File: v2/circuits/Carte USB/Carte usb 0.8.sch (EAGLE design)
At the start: 15 parts, among them Q1 TIP31C, Q2 TIP31C, Q3 TIP31C, Q4 TIP30, Q5 TIP30, Q6 TIP30, X1 MKS1854-6-0-404, X2 MKS1854-6-0-404, X3 MKS1854-6-0-404

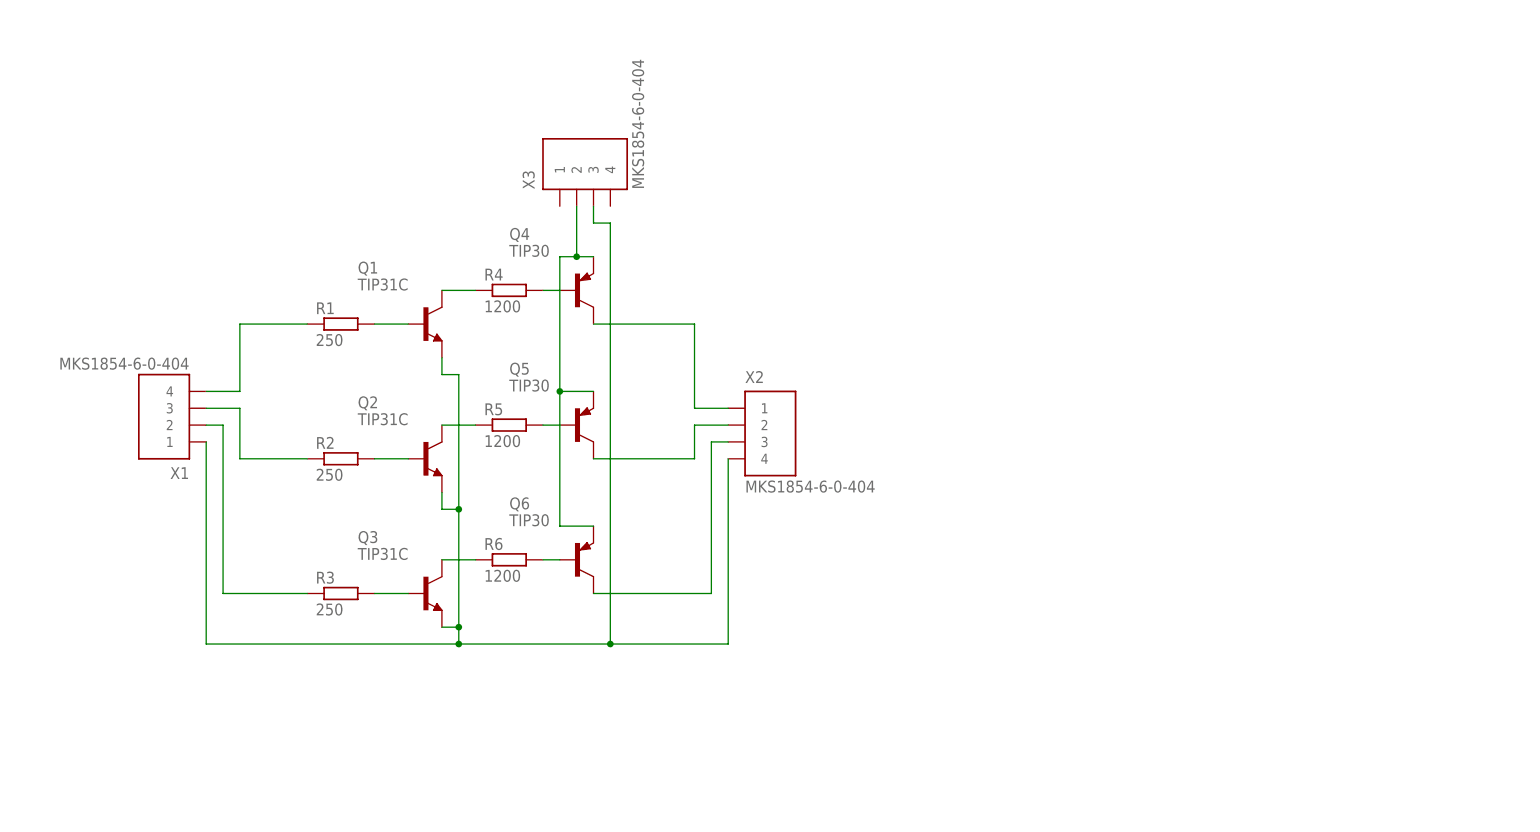
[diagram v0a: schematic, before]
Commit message: added boards
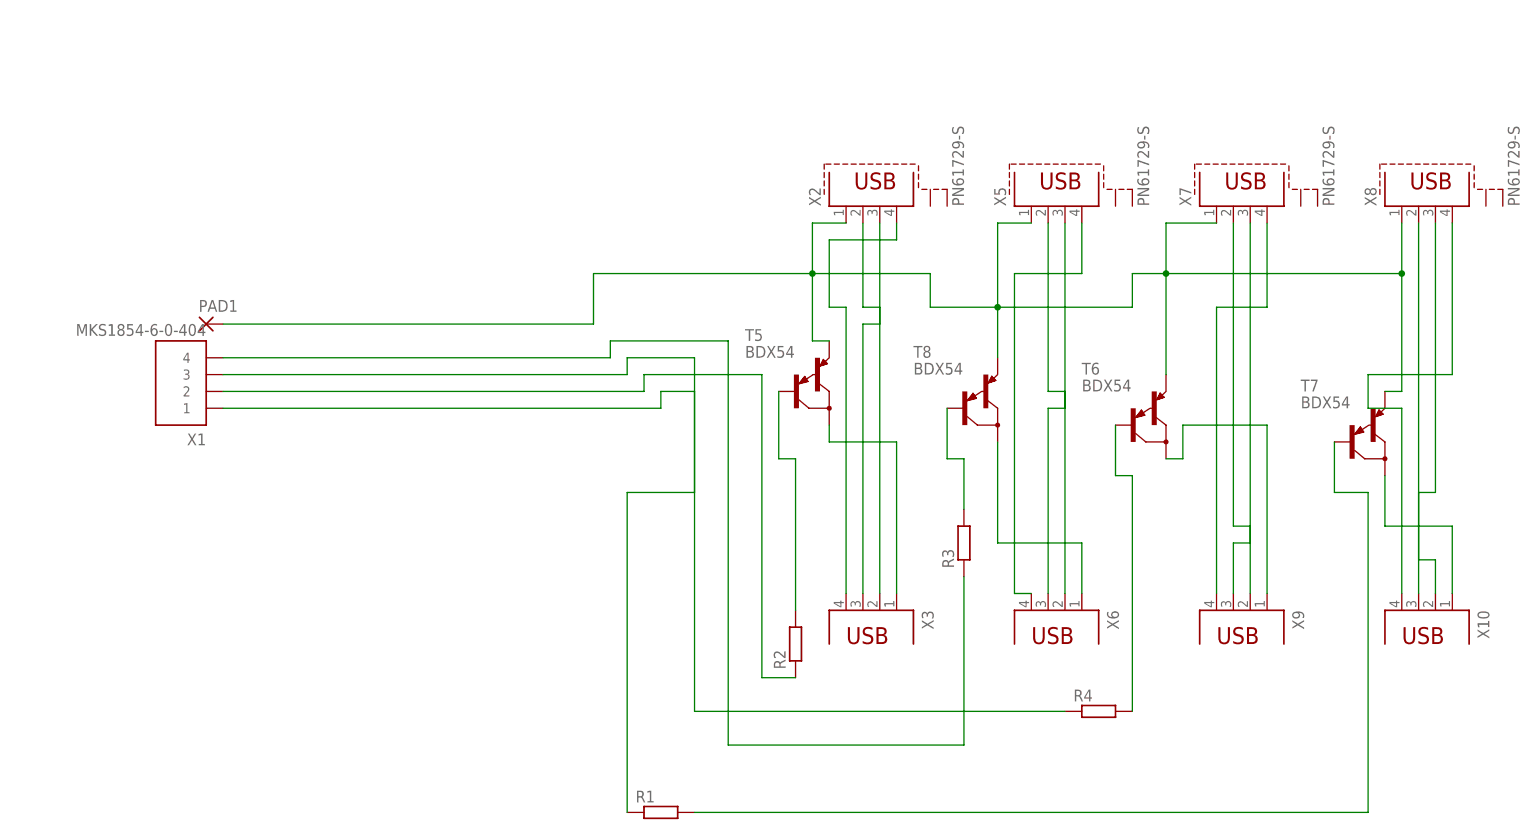
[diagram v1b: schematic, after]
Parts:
- removed Q1, Q2, Q3: TIP31C, transistor-npn:TIP31C
- removed Q4, Q5, Q6: TIP30, transistor-pnp:TIP30
- removed R5, R6: 1200, resistor:R-EU_0207/10
- added PAD1: (no value), wirepad:2,54/1,1
- added T5, T6, T7, T8: BDX54, transistor:BDX54
- added X10, X6, X9: (no value), con-berg:PN87520
- added X5, X7, X8: PN61729-S, con-berg:PN61729-S
- R1, R2, R3: value 250 -> (none); device resistor:R-EU_0207/10 -> rcl:R-EU_0207/10
- R4: value 1200 -> (none); device resistor:R-EU_0207/10 -> rcl:R-EU_0207/10
- X2: value MKS1854-6-0-404 -> PN61729-S; device con-stocko:MKS1854-6-0-404 -> con-berg:PN61729-S
- X3: value MKS1854-6-0-404 -> (none); device con-stocko:MKS1854-6-0-404 -> con-berg:PN87520
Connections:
- removed net N$3: Q3.B, R3.2
- removed net N$6: Q3.C, R6.1
- new net N$19: X5.4, X6.4
- new net N$20: T6.C, X9.1
- new net N$21: T7.C, X10.1
- new net N$22: X7.4, X9.4
- new net N$25: T5.C, X3.1
- new net N$29: R1.2, T7.B
- new net N$30: R1.1, X1.1
- new net N$31: R2.1, X1.2
- new net N$32: R4.1, X1.3
- new net N$33: R3.1, X1.4
- net N$1: now also R2.2, T5.B; no longer Q1.B, R1.2
- net N$10: now also X5.2, X6.2; no longer Q1.E, Q2.E, Q3.E, X1.1, X2.4, X3.3
- net N$12: now also X7.2, X9.2; no longer R1.1, X1.4
- net N$13: now also X2.4, X3.4; no longer R2.1, X1.3
- net N$14: now also X7.3, X9.3; no longer R3.1, X1.2
- net N$15: now also PAD1.P, T5.E, T6.E, T7.E, T8.E, X2.1, X5.1, X7.1, X8.1; no longer Q4.E, Q5.E, Q6.E, X3.2
- net N$16: now also X10.2, X8.2; no longer Q4.C, X2.1
- net N$17: now also X10.3, X8.3; no longer Q5.C, X2.2
- net N$18: now also X10.4, X8.4; no longer Q6.C, X2.3
- net N$2: now also R3.2, T8.B; no longer Q2.B, R2.2
- net N$4: now also X2.2, X3.2; no longer Q1.C, R4.1
- net N$5: now also R4.2, T6.B; no longer Q2.C, R5.1
- net N$7: now also X2.3, X3.3; no longer Q4.B, R4.2
- net N$8: now also X5.3, X6.3; no longer Q5.B, R5.2
- net N$9: now also T8.C, X6.1; no longer Q6.B, R6.2
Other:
- moved on the sheet: R1, R2, R3, R4, X1, X3
